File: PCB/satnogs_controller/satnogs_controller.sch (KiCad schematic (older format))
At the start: 57 parts, among them P1 DEV-PINS, P2 End-Stops, P3 RJ45, P4 I2C, P7 Motor1, P8 Motor2, U1 ARDUINO_PRO_MINI, U2 MAX485, U3 POLOLU_A4988, U4 POLOLU_A4988, U5 TPS54360DDA, U6 POLOLU_DUAL_MC33926, U7 PCA9540B

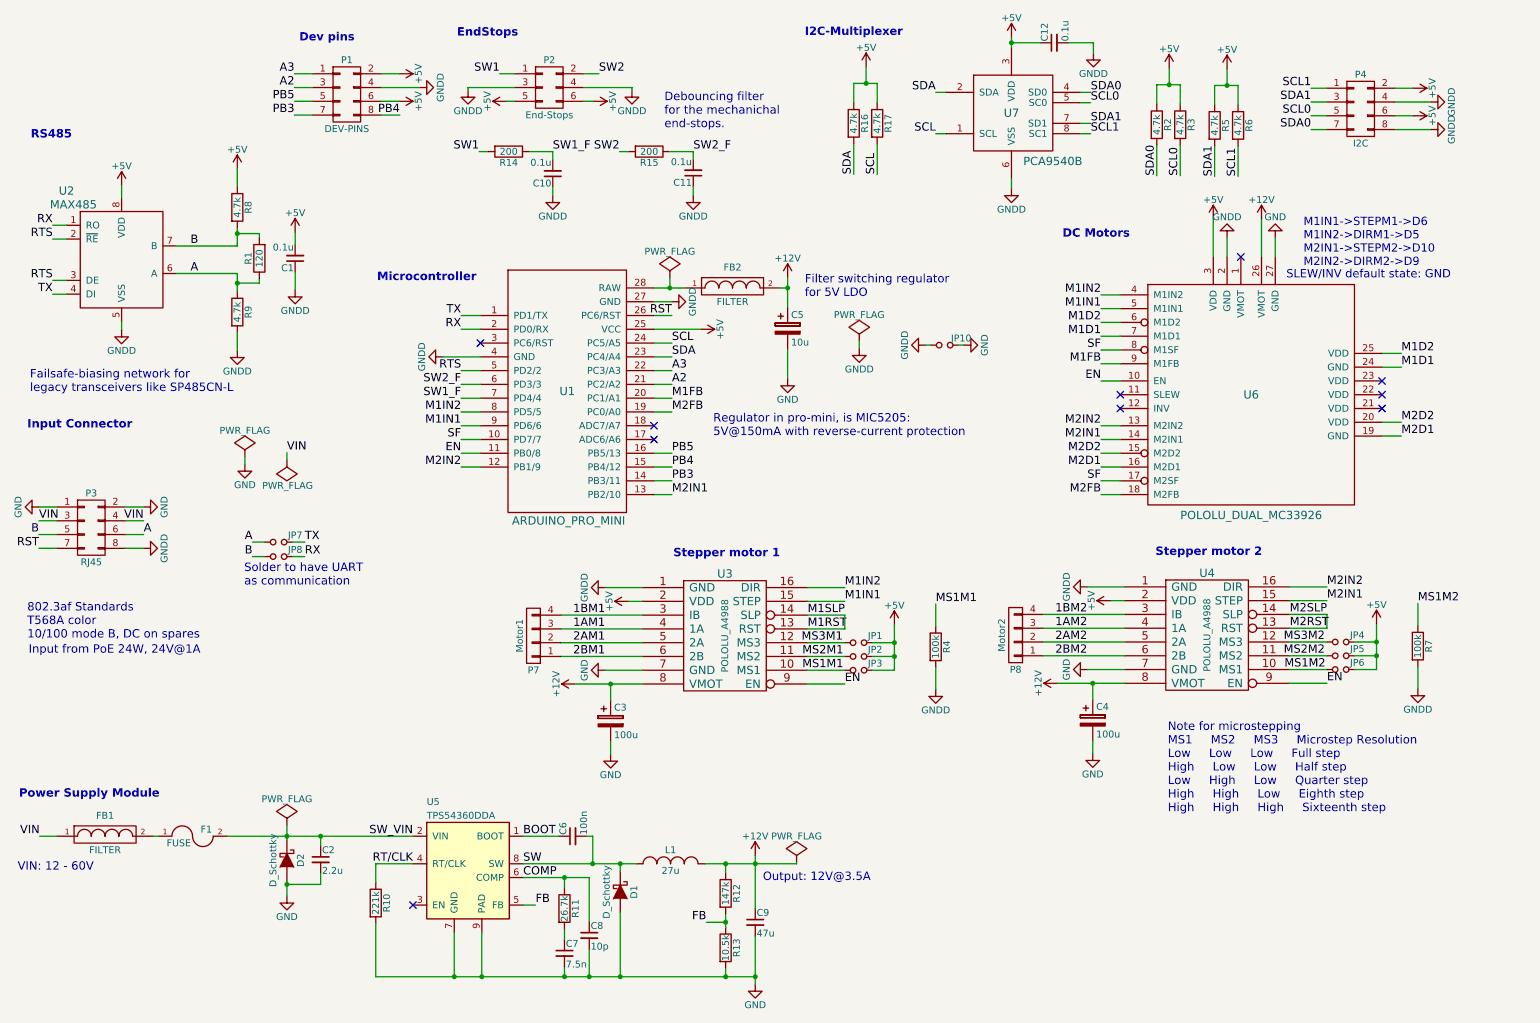
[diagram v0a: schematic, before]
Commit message: wip
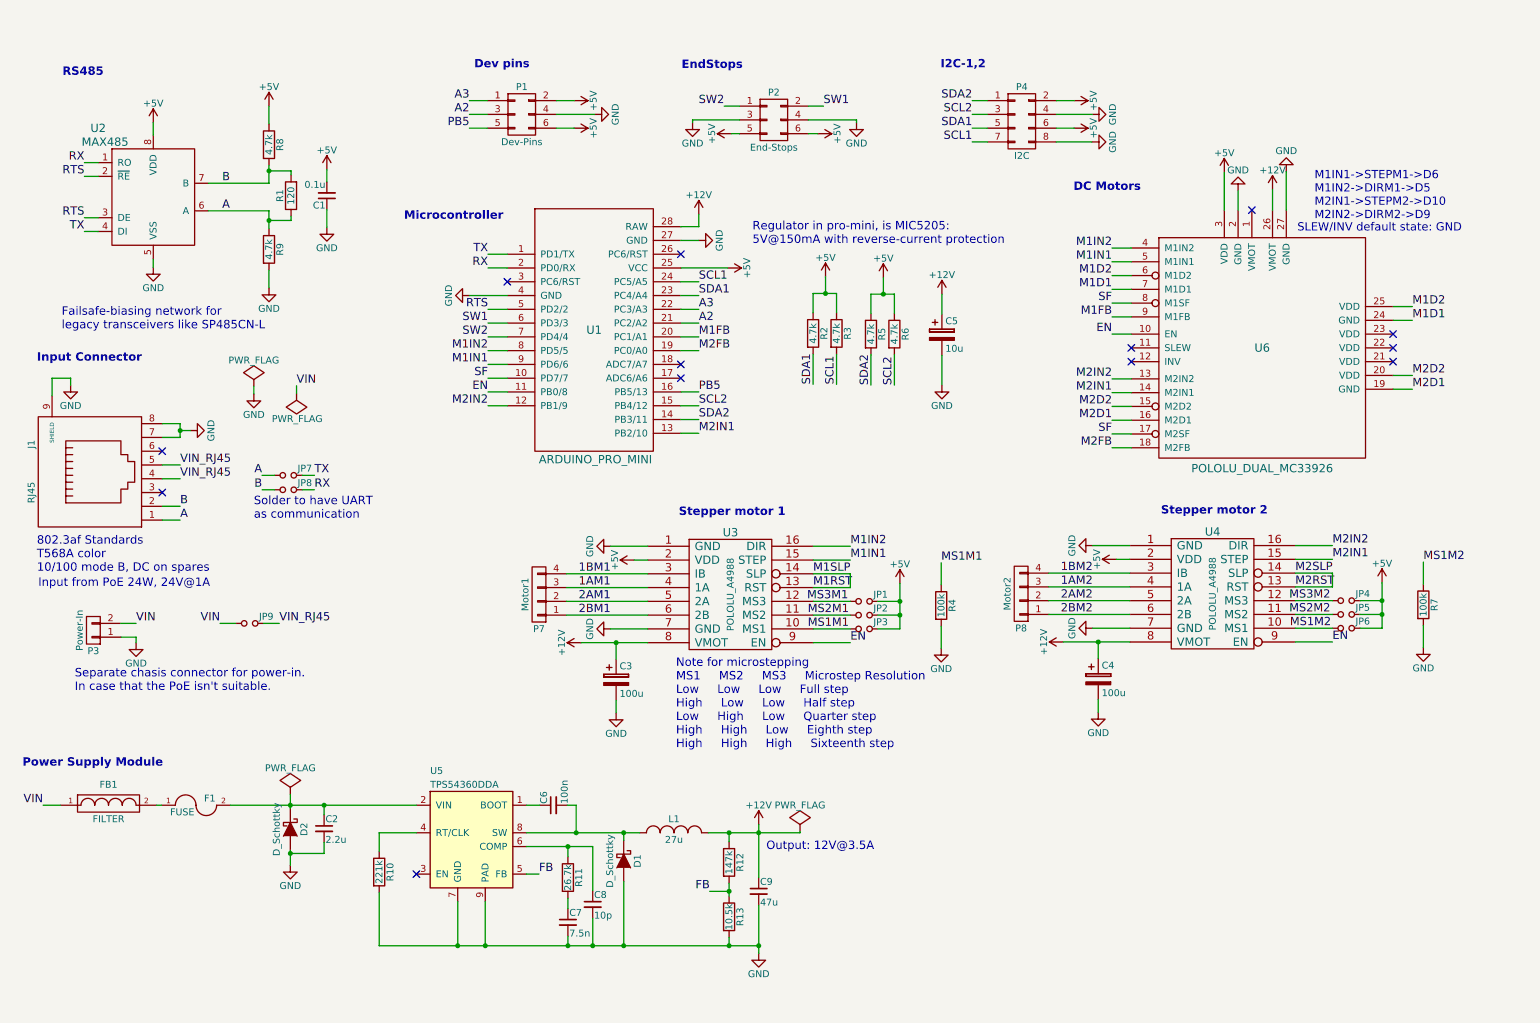
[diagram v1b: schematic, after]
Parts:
- removed C10, C11, C12: 0.1u, Capacitors_SMD:C_0805_HandSoldering, symbol C_Small
- removed FB2: FILTER, Resistors_SMD:R_0805_HandSoldering, symbol FILTER
- removed JP10: Jumper_NO_Small, Resistors_SMD:R_0805_HandSoldering, symbol Jumper_NO_Small
- removed P1: DEV-PINS, Pin_Headers:Pin_Header_Straight_2x04, symbol CONN_02X04
- removed P3: RJ45, Pin_Headers:Pin_Header_Straight_2x04, symbol CONN_02X04
- removed R14, R15: 200, Resistors_SMD:R_0805_HandSoldering, symbol R
- removed R16, R17: 4.7k, Resistors_SMD:R_0805_HandSoldering, symbol R
- removed U7: PCA9540B, Housings_SSOP:TSSOP-8_3x3mm_Pitch0.65mm, symbol PCA9540B
- added J1: RJ45, Connect:RJ45_8, symbol RJ45
- added JP9: Jumper_NO_Small, Resistors_SMD:R_0805_HandSoldering, symbol Jumper_NO_Small
- added P1: Dev-Pins, Pin_Headers:Pin_Header_Straight_2x03, symbol CONN_02X03
- added P3: Power-In, Wire_Connections_Bridges:WireConnection_2.00mmDrill, symbol CONN_01X02
- C1: Distributor (none) -> Mouser 77-VJ0805Y104KXJCBC; Manufacturer (none) -> VJ0805Y104KXJCW1BC; Mnf. VJ0805Y104KXJCW1BC -> (none); Notes (none) -> 16VDC; Package (none) -> 0805; Price 0.118 -> 0.118€
- C2: Mnf. C3225X7R2A225K230AB -> (none); Price 0.697 -> (none)
- C3, C4: footprint Capacitors_SMD:c_elec_6.3x5.3 -> Capacitors_ThroughHole:C_Radial_D6.3_L11.2_P2.5; Distributor (none) -> Mouser 667-ECA-1VM101; Manufacturer (none) -> ECA-1VM101; Mnf. EXV107M016A9GAA -> (none); Notes (none) -> 100u 35V 85C; Package (none) -> ThroughHole:C_Radial_D6.3_L11.2_P2.5; Price 0.443 -> 0.235€
- C5: footprint Capacitors_SMD:c_elec_6.3x5.3 -> Capacitors_ThroughHole:C_Radial_D6.3_L11.2_P2.5; Distributor (none) -> Mouser 667-ECA-1EM100B; Manufacturer (none) -> ECA-1EM100B; Mnf. EXV107M016A9GAA -> (none); Notes (none) -> 10uF 25VDC 85C; Package (none) -> ThroughHole:C_Radial_D6.3_L11.2_P2.5; Price 0.443 -> 0.136€
- C6: Mnf. 08053C104KAT2A -> (none); Price 0.091 -> (none)
- C7: Mnf. GRM2195C1H752JA01D -> (none); Price 0.244 -> (none)
- C8: Mnf. C0805C100K5GACTU -> (none); Price 0.091 -> (none)
- C9: Mnf. GRM32ER61C476ME15L -> (none); Price 0.851 -> (none)
- D1, D2: Mnf. B560C-13-F -> (none); Price 0.494 -> (none)
- F1: footprint satnogs:mini-fuse-holder-3568 -> SMD_Packages:Fuse_SMD; Mnf. Keystone Electronics, 3568 -> (none); Price 0.732 -> (none)
- FB1: Mnf. MPZ2012S300A -> (none); Price 0.109 -> (none)
- JP1, JP2, JP3, JP4, JP5, JP6, JP7, JP8: Distributor (none) -> SparkFun PRT-12791; Manufacturer (none) -> -; Notes (none) -> https://www.sparkfun.com/products/12791; Package (none) -> 2x23 pin male PTH header; Price (none) -> -
- L1: Mnf. SRR1210-270M -> (none); Price 1 -> (none)
- P7, P8: Distributor (none) -> SparkFun PRT-08432; Manufacturer (none) -> -; Mnf. Altech - 30.704 -> (none); Notes (none) -> https://www.sparkfun.com/products/8432; Package (none) -> 5mm Pitch 4-Pin; Price 1.99 -> 1.8€
- R1: Distributor (none) -> Mouser 71-CRCW0805120RJNEA; Manufacturer (none) -> CRCW0805120RJNEA; Mnf. CRCW0805120RJNEA -> (none); Notes (none) -> 1/8W 5%; Package (none) -> 0805; Price 0.091 -> 0.091€
- R10: Mnf. CRCW0805221KFKEA -> (none); Price 0.091 -> (none)
- R11: Mnf. CRCW080526K7FKEA -> (none); Price 0.091 -> (none)
- R12: Mnf. CRCW0805147KFKEA -> (none); Price 0.091 -> (none)
- R13: Mnf. CRCW080510K5FKEA -> (none); Price 0.091 -> (none)
- R2, R3, R5, R6, R8: Distributor (none) -> Mouser 71-CRCW0805J-4.7K-E3; Manufacturer (none) -> CRCW08054K70JNEA; Mnf. CRCW08054K70JNEA -> (none); Notes (none) -> 1/8W 5%; Package (none) -> 0805; Price 0.091 -> 0.091€
- R4: Distributor (none) -> Mouser 71-CRCW0805J-100K-E3; Manufacturer (none) -> CRCW0805100KJNEA; Mnf. CRCW0805100KJNEA -> (none); Package (none) -> 0805; Price 0.091 -> 0.091€
- R7: Distributor (none) -> Mouser 71-CRCW0805J-100K-E3; Manufacturer (none) -> CRCW0805100KJNEA; Mnf. CRCW0805100KJNEA -> (none); Notes (none) -> 1/8W 5%; Package (none) -> 0805; Price 0.091 -> 0.091€
- R9: Distributor (none) -> Mouser 71-CRCW0805J-4.7K-E3; Notes (none) -> 1/8W 5%; Package (none) -> 0805; Price 0.091 -> 0.091€
- U1: Mnf. Sparkfun - DEV-11113 -> (none); Price 9.5 -> (none)
- U2: Distributor (none) -> Mouser 701-SP485CN-L; Notes (none) -> Operating Supply Voltage: 5 V; Package (none) -> SOIC-8 Narrow; Price 0.86 -> 0.86€
- U3: Distributor (none) -> SparkFun PRT-00115; Manufacturer (none) -> -; Mnf. 1182 -> (none); Notes (none) -> https://www.sparkfun.com/products/115; Package (none) -> 1x40 female header PTH pitch 2.54; Price 5.95 -> 1.42€
- U4: Distributor (none) -> SparkFun PRT-00115; Manufacturer (none) -> -; Mnf. 1182 -> (none); Notes (none) -> https://www.sparkfun.com/products/115; Package (none) -> 1x40 female header PTH pitch 2.54; Price 5.95 -> -
- U5: Mnf. TPS54360DDAR -> (none); Price 4.53 -> (none)
- U6: Mnf. 1213 -> (none); Price 27.83 -> (none)
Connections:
- net GNDD is gone; now on net GND: C1.1, P2.3 (P3), P2.4 (P4), P4.4 (P4), P4.8 (P8), R4.2, R7.2, R9.2, U1.27 (GND), U1.4 (GND), U2.5 (VSS), U3.1 (GND), U4.1 (GND), U6.2 (GND)
- net SCL is gone; now on net SCL1: U1.24 (PC5/A5)
- net SDA is gone; now on net SDA1: U1.23 (PC4/A4)
- net SW1_F is gone; now on net SW2: U1.7 (PD4/4)
- net SW2_F is gone; now on net SW1: U1.6 (PD3/3)
- net +12V: now also U1.28 (RAW)
- net +5V: now also P1.2 (P2), P1.6 (P6)
- net A: now also J1.1
- net A2: now also P1.3 (P3)
- net A3: now also P1.1 (P1)
- net B: now also J1.2
- net GND: now also J1.7, J1.8, J1.9 (SHIELD), P1.4 (P4), P3.1 (P1)
- net PB5: now also P1.5 (P5)
- net SCL1: now also P4.7 (P7), R3.2; no longer P4.1 (P1), R6.2
- net SDA1: now also P4.5 (P5), R2.2; no longer P4.3 (P3), R5.2
- net SW1: now also P2.2 (P2); no longer P2.1 (P1)
- net SW2: now also P2.1 (P1); no longer P2.2 (P2)
- net VIN: now also JP9.1, P3.2 (P2)
- net BOOT: no longer names the net of C6.1, U5.1 (BOOT)
- net COMP: no longer names the net of C8.1, R11.1, U5.6 (COMP)
- net PB3 renamed SDA2
- net SDA2: now also P4.1 (P1), R5.2
- net PB4 renamed SCL2
- net SCL2: now also P4.3 (P3), R6.2
- net RST: no longer names the net of U1.26 (PC6/RST)
- net RT/CLK: no longer names the net of R10.1, U5.4 (RT/CLK)
- removed net SCL0: P4.5 (P5), R3.2
- removed net SDA0: P4.7 (P7), R2.2
- net SW: no longer names the net of C6.2, D1.1 (K), L1.1, U5.8 (SW)
- net SW_VIN: no longer names the net of C2.1, D2.1 (K), F1.2, U5.2 (VIN)
- new net VIN_RJ45: J1.4, J1.5, JP9.2
- no-connect marks 10 -> 13
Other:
- note added: "I2C-1,2"
- note added: "Separate chasis connector for power-in.\nIn case that the PoE isn't suitable."
- note removed: "Debouncing filter\nfor the mechanichal\nend-stops.\n"
- note removed: "Filter switching regulator\nfor 5V LDO"
- note removed: "I2C-Multiplexer"
- note removed: "VIN: 12 - 60V"
- moved on the sheet: C1, C2, C3, C4, C5, C6, C7, C8, C9, D1, D2, F1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
